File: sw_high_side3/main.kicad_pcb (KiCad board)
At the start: 2 copper layers, 11 parts, among them P1 CONN_01X02, P2 CONN_02X03, P3 CONN_01X02, P4 CONN_XT60, P5 CONN_XT60, Q1 IRFB7537PbF, U1 NSI45020AT1G, U2 MIC5014, U3 74LVC1G08

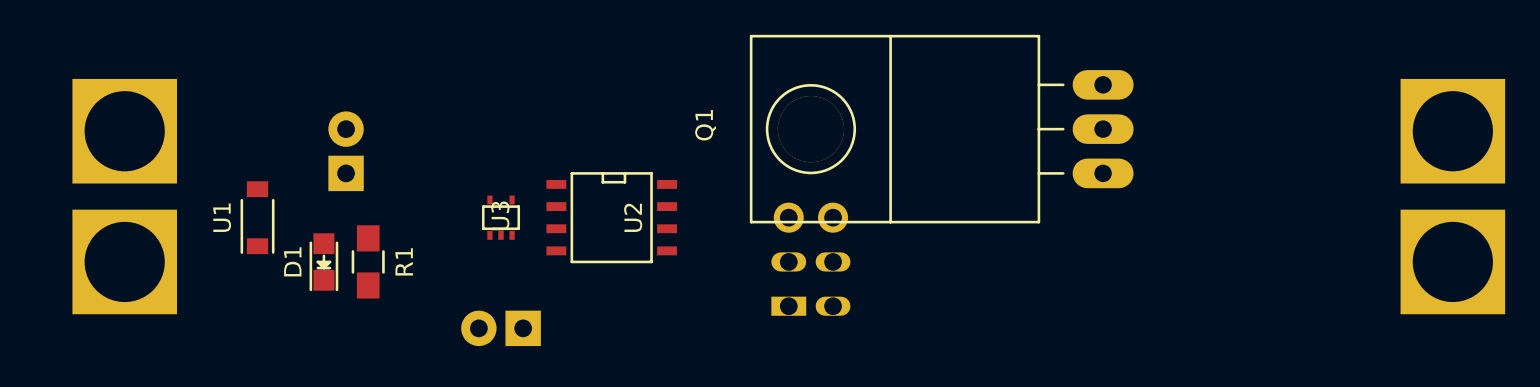
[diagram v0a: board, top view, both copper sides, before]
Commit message: test
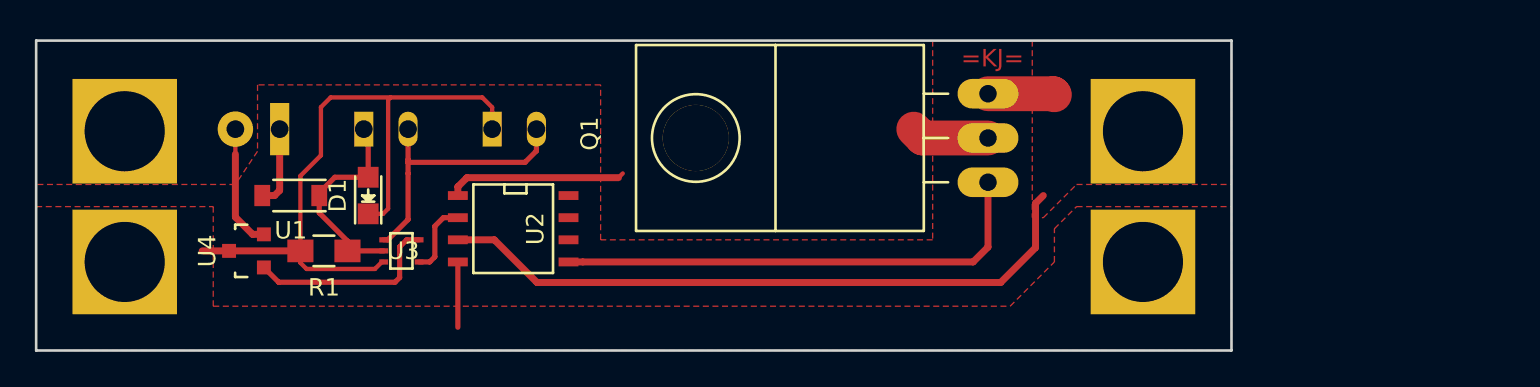
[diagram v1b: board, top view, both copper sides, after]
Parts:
- added U4: LM3480-3.3, TO_SOT_Packages_SMD:SOT-23, F.Cu at (108.6, 90.8)
- P2: value CONN_02X03 -> CONN_01X02; footprint Pin_Headers:Pin_Header_Straight_2x03 -> Pin_Headers:Pin_Header_Straight_1x02
- moved P2 19.8 mm to (122.7, 83.8), turned to 270 degrees
- moved P5 17.8 mm to (160.0, 91.4)
- moved P3 14.6 mm to (115.3, 83.8), turned to 270 degrees
- moved Q1 6.62 mm to (151.1, 84.3)
- moved U3 6.02 mm to (117.5, 90.8), turned to 0 degrees
- moved U2 5.69 mm to (123.9, 89.5)
- moved P1 4.58 mm to (110.5, 83.8), turned to 90 degrees
- moved D1 4.58 mm to (115.6, 87.6)
- moved R1 2.62 mm to (113.0, 90.8), turned to 180 degrees
- moved U1 2.29 mm to (111.1, 87.6), turned to 180 degrees
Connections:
- U3 pad 5: Net-(D1-Pad2) -> Net-(U3-Pad5)
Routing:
- net /In-: track 0.00 -> 43.2 mm
- net /Out+: track 0.00 -> 42.0 mm
- net Net-(Q1-Pad1): track 0.00 -> 28.1 mm
- net /In+: track 0.00 -> 21.8 mm
- net Net-(P2-Pad2): track 0.00 -> 16.3 mm
- net Net-(D1-Pad2): track 0.00 -> 12.1 mm
- net Net-(U3-Pad5): track 0.00 -> 11.3 mm
- net Net-(P1-Pad1): track 0.00 -> 4.64 mm
- net Net-(U2-Pad2): track 0.00 -> 4.30 mm
- added copper zone on F.Cu, net /In+
- added copper zone on F.Cu, net /In-
- added copper zone on F.Cu, net /Out+
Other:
- board outline added: 68.6 x 17.8 mm
- board text added: "=KJ="
